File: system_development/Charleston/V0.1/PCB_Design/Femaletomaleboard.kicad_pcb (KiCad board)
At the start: 2 copper layers, 56.3 x 32.8 mm, 3 parts, among them SW2 MC74VHC1G66DFT1G

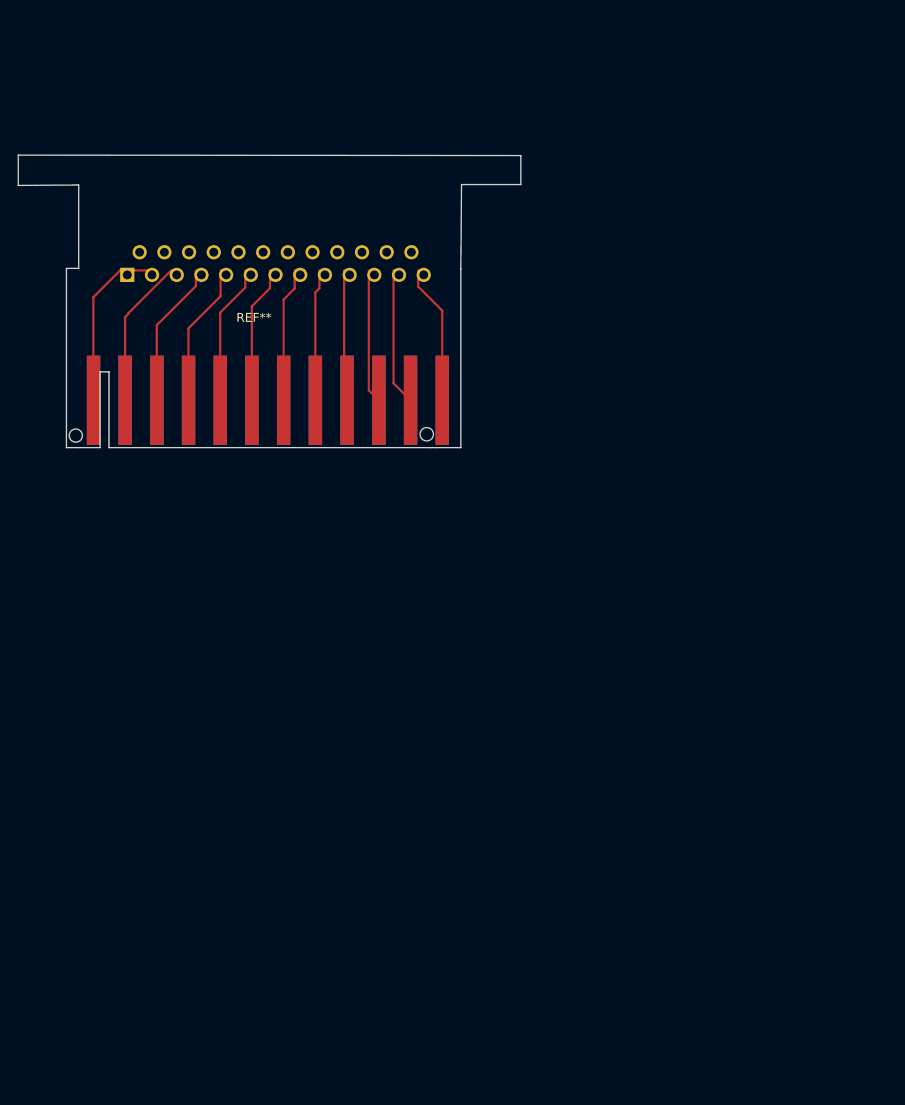
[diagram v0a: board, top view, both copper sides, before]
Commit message: Female to male board
3rd times the charm
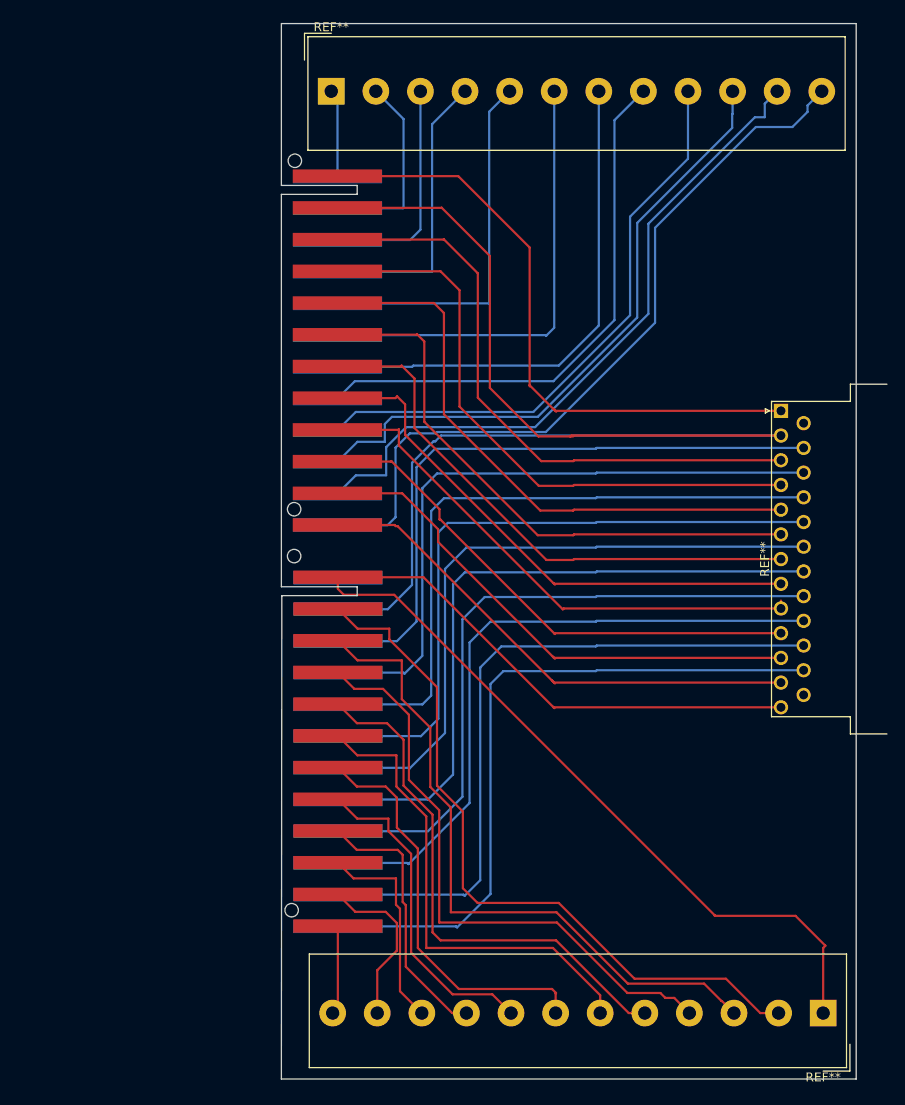
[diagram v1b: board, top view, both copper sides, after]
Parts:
- removed the REF** at (94.4, 70.6)
- removed the SW2 at (110.1, 79.0)
- removed the SW2 at (112.2, 79.0)
- added REF**: Altech_AK300_1x12_P5.00mm_45-Degree, TerminalBlock_Altech:Altech_AK300_1x12_P5.00mm_45-Degree, F.Cu at (117.2, 50.0)
- added REF**: DSUB-25_Female_Horizontal_P2.77x2.54mm_EdgePinOffset9.40mm, Connector_Dsub:DSUB-25_Female_Horizontal_P2.77x2.54mm_EdgePinOffset9.40mm, F.Cu at (167.7, 85.8)
- added REF**: Altech_AK300_1x12_P5.00mm_45-Degree, TerminalBlock_Altech:Altech_AK300_1x12_P5.00mm_45-Degree, F.Cu at (172.4, 153.3)
- added SW2: MC74VHC1G66DFT1G, infnoise_goldfingers:Gold Finger PCB, F.Cu at (123.6, 124.0)
- added SW2: MC74VHC1G66DFT1G, infnoise_goldfingers:Gold Finger PCB, F.Cu at (123.5, 79.1)
- added SW2: MC74VHC1G66DFT1G, infnoise_goldfingers:Gold Finger PCB bottom, B.Cu at (123.6, 126.1)
- added SW2: MC74VHC1G66DFT1G, infnoise_goldfingers:Gold Finger PCB bottom, B.Cu at (112.4, 77.1)
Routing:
- net (no net): track 191.3 -> 2812.8 mm
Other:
- board size 56.3 x 32.8 mm -> 64.4 x 118.3 mm
